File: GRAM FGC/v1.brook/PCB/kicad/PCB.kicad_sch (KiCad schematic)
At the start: 24 parts, among them J1 USB_C_Receptacle_USB2.0_16P, SW1 SW_Push, SW2 SW_Push, SW3 SW_Push, SW4 SW_Push

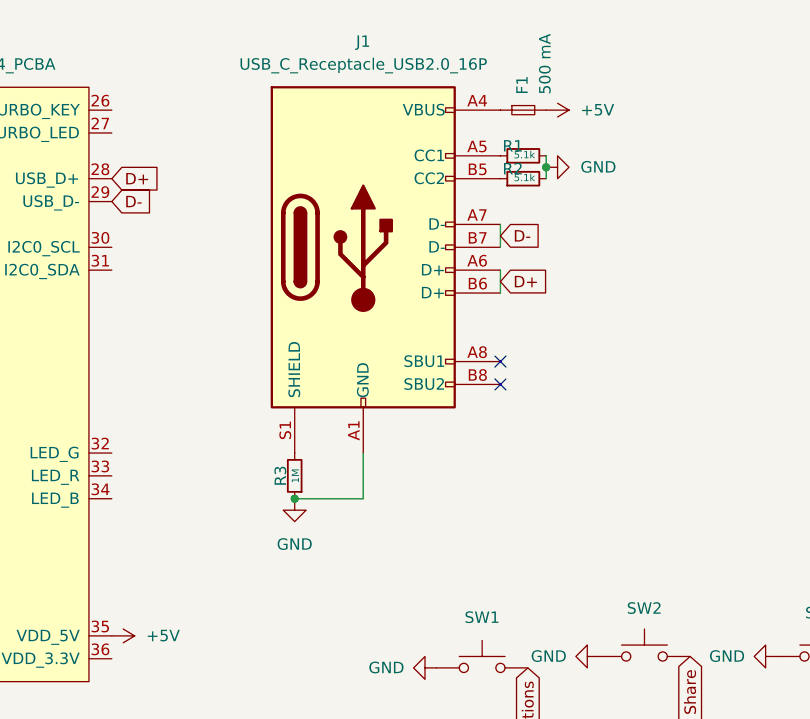
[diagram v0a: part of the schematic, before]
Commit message: Final working version
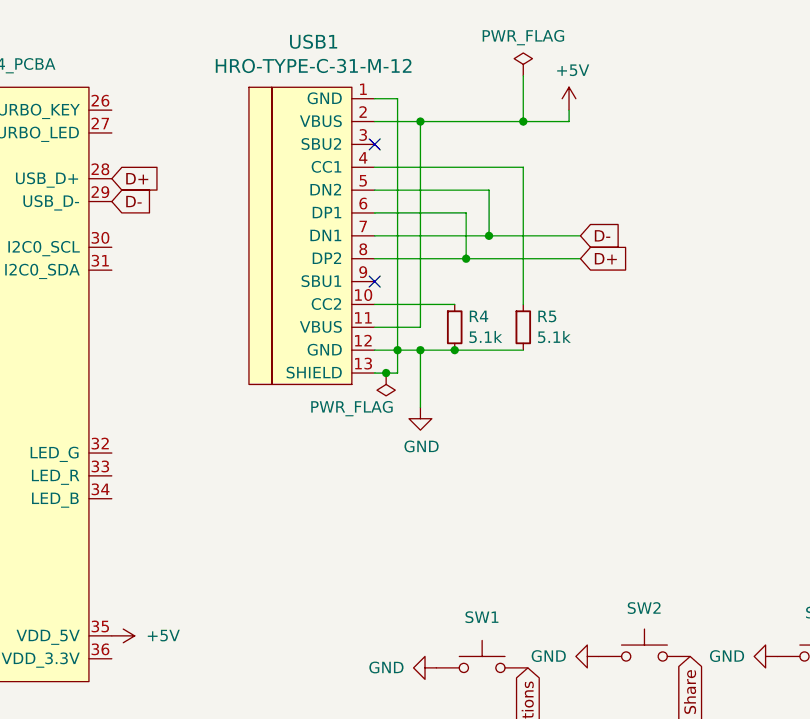
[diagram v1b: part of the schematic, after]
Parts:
- removed F1: 500 mA, Fuse:Fuse_1206_3216Metric, symbol Device:Fuse_Small
- removed J1: USB_C_Receptacle_USB2.0_16P, PCM_marbastlib-xp-various:USB_C_Receptacle_HRO_TYPE-C-31-M-23, symbol Connector:USB_C_Receptacle_USB2.0_16P
- removed R1, R2: 5.1k, Resistor_SMD:R_0402_1005Metric, symbol Device:R_Small
- removed R3: 1M, Resistor_SMD:R_0603_1608Metric, symbol Device:R_Small
- added R4, R5: 5.1k, Resistor_SMD:R_0805_2012Metric, symbol Device:R_Small
- added USB1: HRO-TYPE-C-31-M-12, Type-C:HRO-TYPE-C-31-M-12, symbol Type-C:HRO-TYPE-C-31-M-12
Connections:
- net +5V: now also USB1.11 (VBUS), USB1.2 (VBUS)
- net D+: now also USB1.6 (DP1), USB1.8 (DP2)
- net D-: now also USB1.5 (DN2), USB1.7 (DN1)
- net GND: now also R4.2, R5.2, USB1.1 (GND), USB1.12 (GND), USB1.13 (SHIELD)
- new net: R4.1, USB1.10 (CC2)
- new net: R5.1, USB1.4 (CC1)
